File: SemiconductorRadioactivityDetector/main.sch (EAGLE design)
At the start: 32 parts, among them IC1 LM324N, IC2 317T, J1 22-05-7028-02, J2 22-23-2021, J3 22-23-2021, J4 22-23-2021, Q1 2N4093

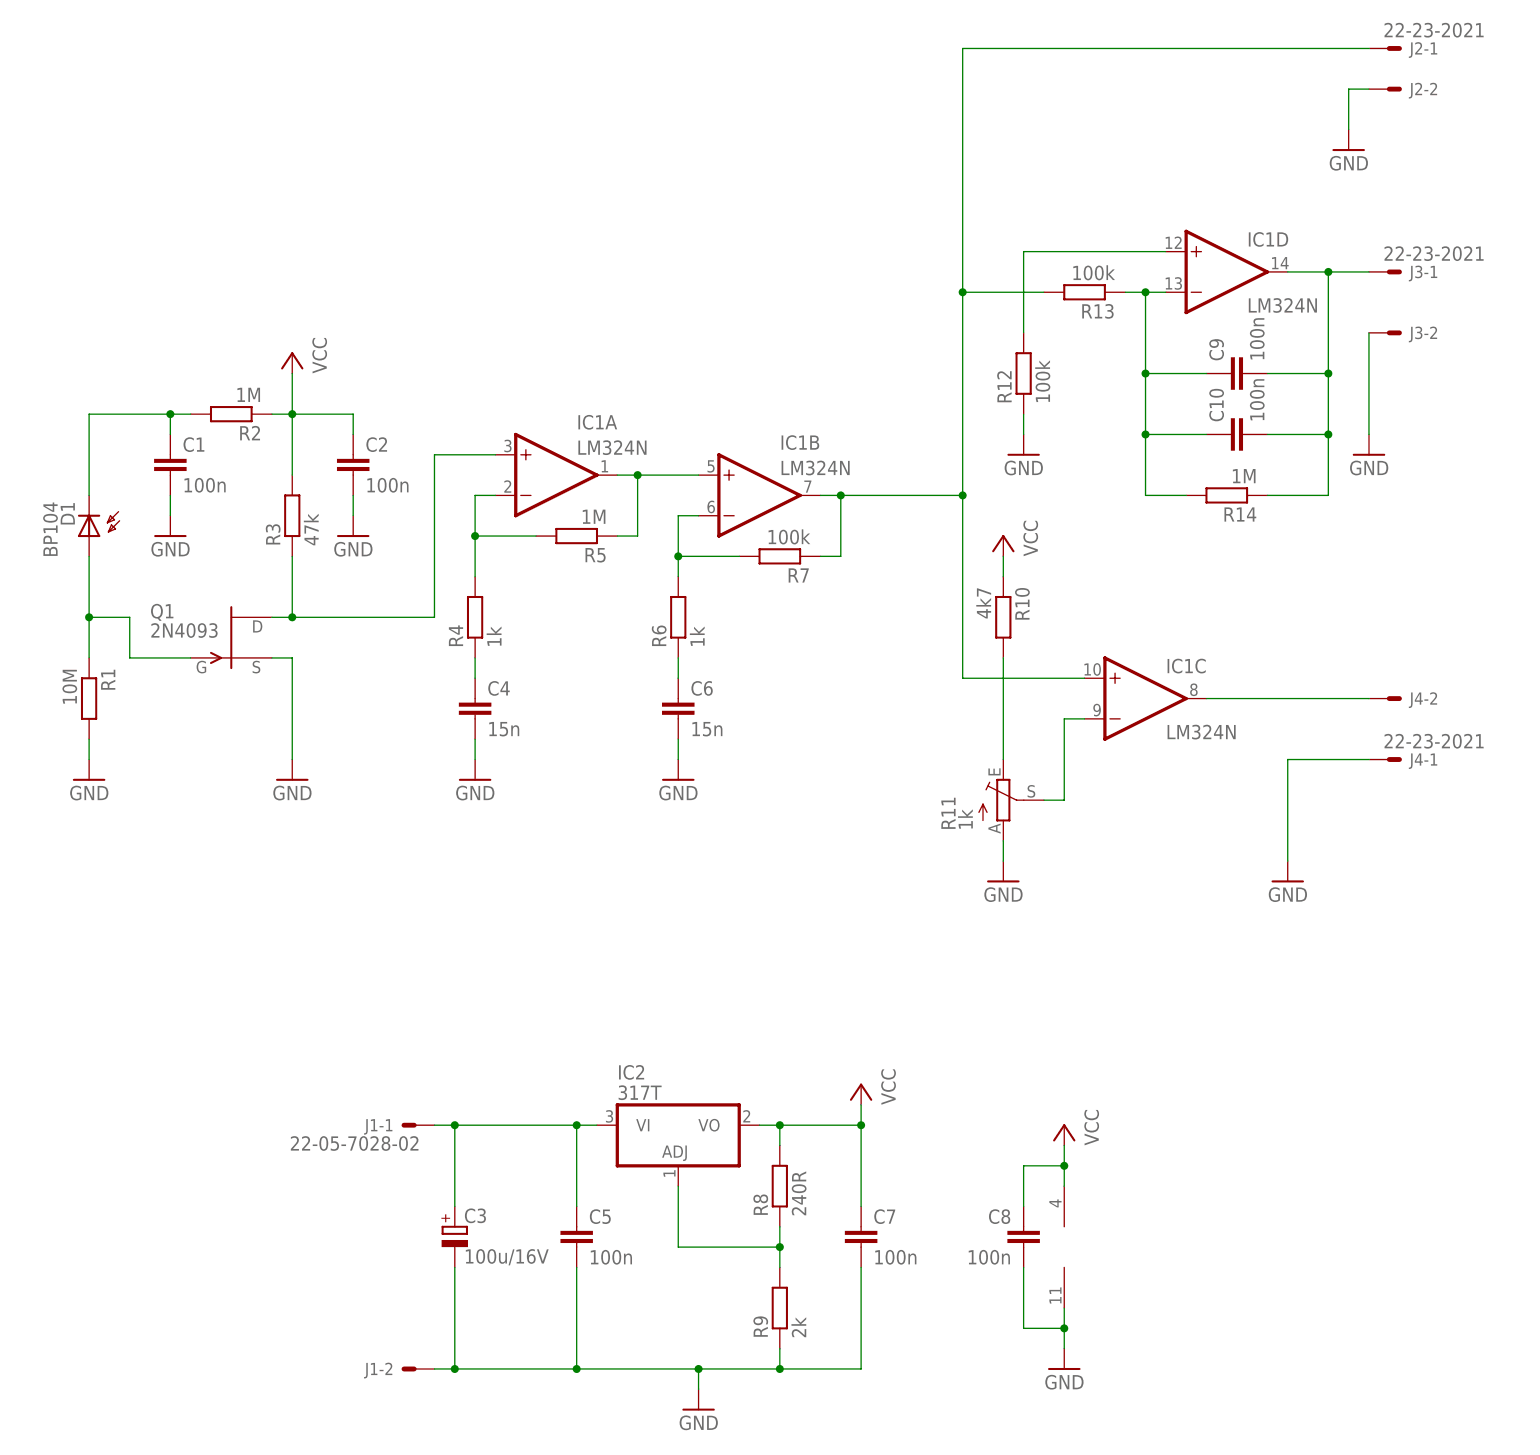
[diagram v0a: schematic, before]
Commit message: Second version. Not working.
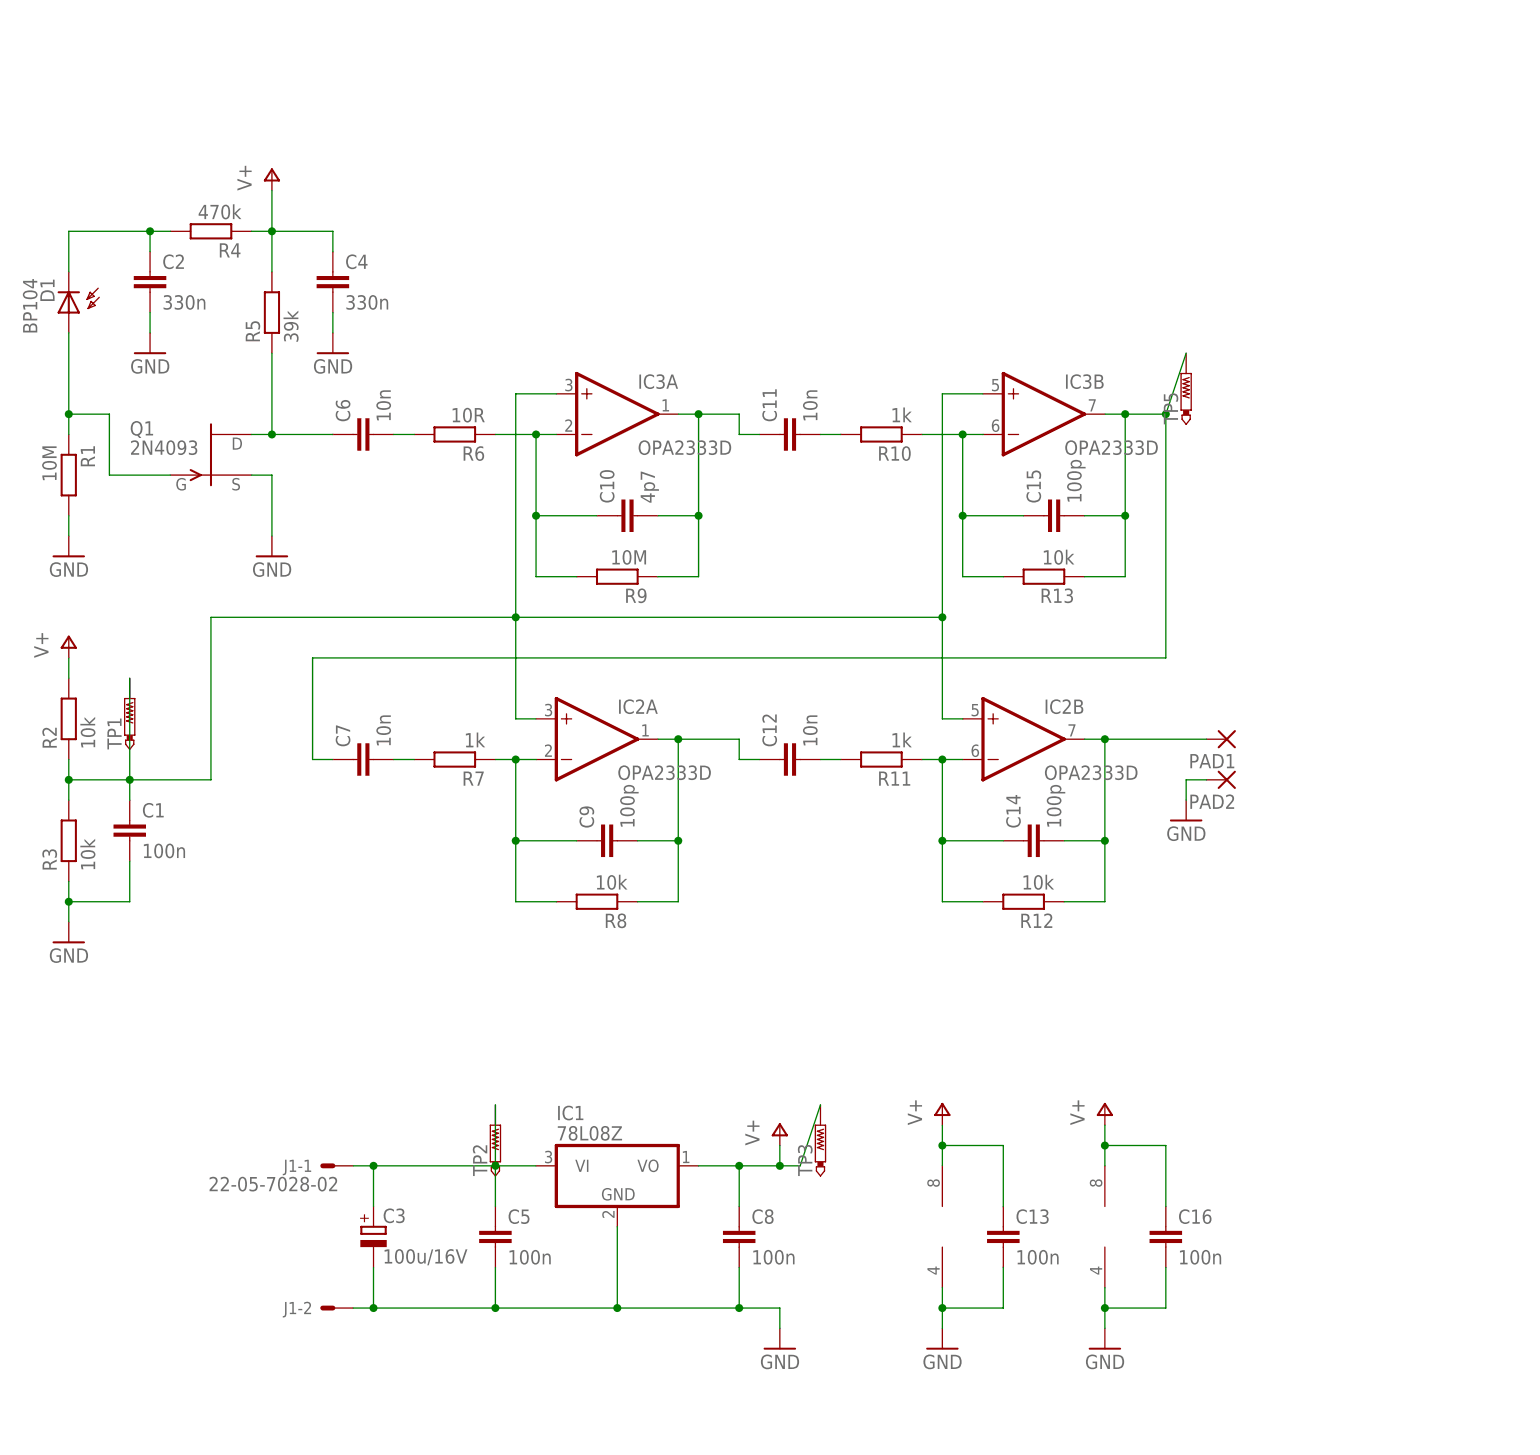
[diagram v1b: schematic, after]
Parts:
- removed J2, J3, J4: 22-23-2021, con-molex:22-23-2021
- removed R14: 1M, resistor:R-EU_M1206
- added C11: 10n, resistor:C-EUC0805
- added C12: 10n, rcl:C-EUC0805
- added C13: 100n, rcl:C-EUC0805
- added C14, C15: 100p, resistor:C-EUC0805
- added C16: 100n, resistor:C-EUC0805
- added IC3: OPA2333D, linear:OPA2333D
- added PAD1, PAD2: (no value), wirepad:1,6/0,8
- added TP1, TP2, TP3, TP5: PTR1TP12R, testpad:PTR1TP12R
- C1, C5, C8: device resistor:C-EUC1206 -> rcl:C-EUC0805
- C10: value 100n -> 4p7; device resistor:C-EUC1206 -> resistor:C-EUC0805
- C2: value 100n -> 330n; device resistor:C-EUC1206 -> rcl:C-EUC0805
- C4: value 15n -> 330n; device resistor:C-EUC1206 -> rcl:C-EUC0805
- C6: value 15n -> 10n; device resistor:C-EUC1206 -> resistor:C-EUC0805
- C7: value 100n -> 10n; device resistor:C-EUC1206 -> resistor:C-EUC0805
- C9: value 100n -> 100p; device resistor:C-EUC1206 -> resistor:C-EUC0805
- IC1: value LM324N -> 78L08Z; device linear:LM324N -> linear:78L08Z
- IC2: value 317T -> OPA2333D; device linear:317T -> linear:OPA2333D
- R10: value 4k7 -> 1k; device resistor:R-EU_M1206 -> rcl:R-EU_R0805
- R11: device pot:TRIM_EU-B64Y -> rcl:R-EU_R0805
- R12: value 100k -> 10k; device resistor:R-EU_R1206 -> rcl:R-EU_R0805
- R13: value 100k -> 10k; device resistor:R-EU_M1206 -> rcl:R-EU_R0805
- R2: value 1M -> 10k; device resistor:R-EU_M1206 -> rcl:R-EU_R0805
- R3: value 47k -> 10k; device resistor:R-EU_M1206 -> rcl:R-EU_R0805
- R4: value 1k -> 470k; device resistor:R-EU_M1206 -> rcl:R-EU_R0805
- R5: value 1M -> 39k; device resistor:R-EU_M1206 -> rcl:R-EU_R0805
- R6: value 1k -> 10R; device resistor:R-EU_M1206 -> rcl:R-EU_R0805
- R7: value 100k -> 1k; device resistor:R-EU_M1206 -> rcl:R-EU_R0805
- R8: value 240R -> 10k; device resistor:R-EU_M1206 -> rcl:R-EU_R0805
- R9: value 2k -> 10M; device resistor:R-EU_M1206 -> rcl:R-EU_0204/2V
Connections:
- removed net N$1: IC2.ADJ, R8.1, R9.2
- removed net N$12: C10.1, C9.1, IC1D.-IN, R13.1, R14.2
- removed net N$18: IC1A.+IN, Q1.D, R3.1
- removed net N$19: IC1B.OUT, IC1C.+IN, J2-1.S, R13.2, R7.1
- removed net N$5: IC1B.-IN, R6.2, R7.2
- removed net VCC: C2.1, C7.1, C8.1, IC1P.V+, IC2.VO, R10.1, R2.1, R3.2, R8.2
- new net N$10: C9.1, IC2A.-IN, R7.1, R8.2
- new net N$20: C10.2, C11.1, IC3A.OUT, R9.1
- new net N$22: C12.1, C9.2, IC2A.OUT, R8.1
- new net N$6: C6.1, Q1.D, R5.1
- new net V+: C13.1, C16.1, C4.1, C8.1, IC1.VO, IC2P.V+, IC3P.V+, R2.2, R4.1, R5.2, TP3.TP
- new net V_REF: C1.1, IC2A.+IN, IC2B.+IN, IC3A.+IN, IC3B.+IN, R2.1, R3.2, TP1.TP
- net GND: now also C13.2, C16.2, IC1.GND, IC2P.V-, IC3P.V-, PAD2.P, R3.1; no longer C6.2, C7.2, IC1P.V-, J2-2.S, J3-2.S, J4-1.S, R11.A, R12.1, R9.1
- net N$11: now also C7.2, R7.2; no longer IC1C.-IN, R11.S
- net N$13: now also C14.1, IC2B.-IN, R11.1, R12.2; no longer C10.2, C9.2, IC1D.OUT, J3-1.S, R14.1
- net N$14: now also C12.2, R11.2; no longer IC1D.+IN, R12.2
- net N$15: now also C11.2, R10.2; no longer IC1C.OUT, J4-2.S
- net N$16: now also C2.1, R4.2; no longer C1.1, R2.2
- net N$2: now also C6.2, R6.2; no longer IC1A.-IN, R4.2, R5.2
- net N$3: now also C14.2, IC2B.OUT, PAD1.P, R12.1; no longer IC1A.OUT, IC1B.+IN, R5.1
- net N$4: now also C10.1, IC3A.-IN, R6.1, R9.2; no longer C4.1, R4.1
- net N$7: now also C15.2, C7.1, IC3B.OUT, R13.1, TP5.TP; no longer C6.1, R6.1
- net N$8: now also IC1.VI, TP2.TP; no longer IC2.VI
- net N$9: now also C15.1, IC3B.-IN, R10.1, R13.2; no longer R10.2, R11.E
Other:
- moved on the sheet: C1, C10, C2, C3, C4, C5, C6, C7, C8, C9, D1, J1-1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

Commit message: Third HW revision, paritialy done.
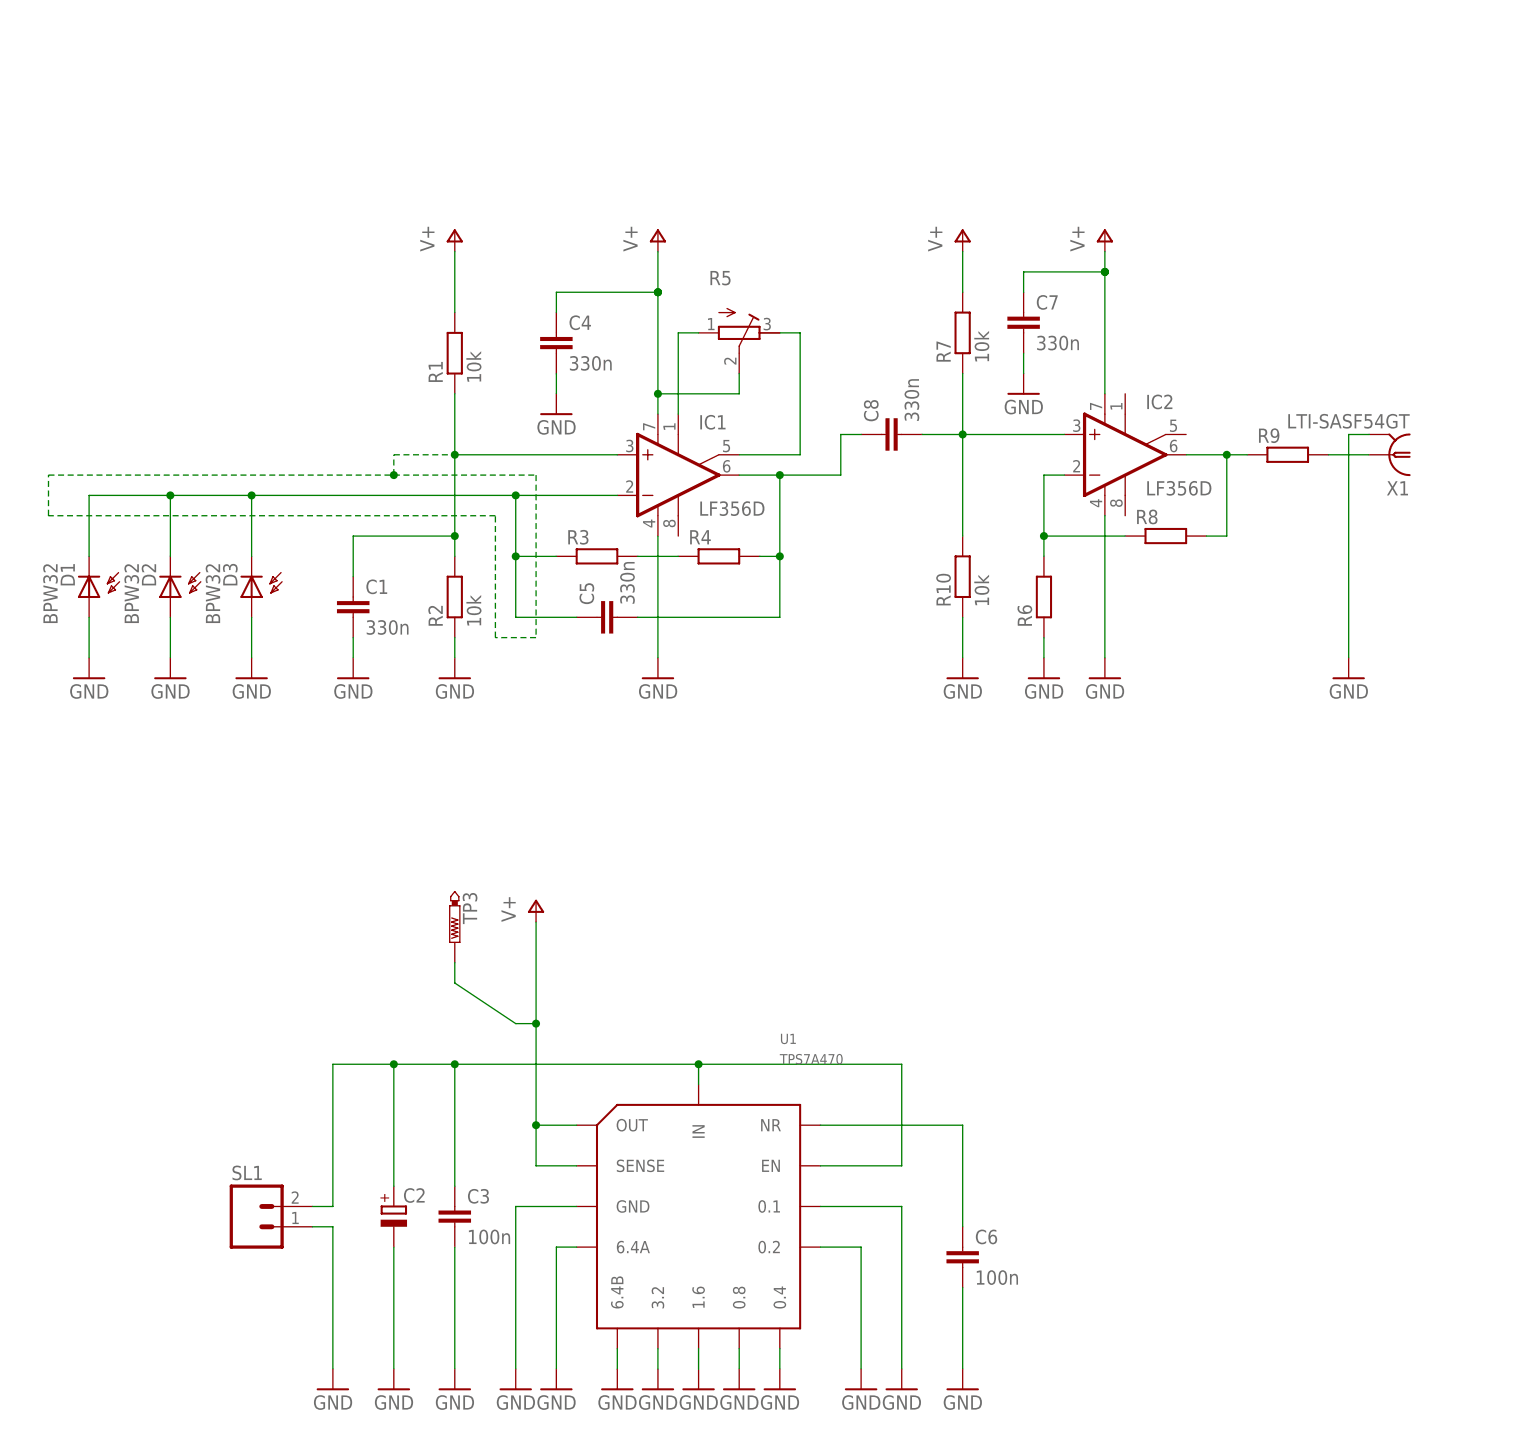
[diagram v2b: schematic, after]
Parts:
- removed C10: 4p7, resistor:C-EUC0805
- removed C11: 10n, resistor:C-EUC0805
- removed C12: 10n, rcl:C-EUC0805
- removed C13: 100n, rcl:C-EUC0805
- removed C14, C15, C9: 100p, resistor:C-EUC0805
- removed C16: 100n, resistor:C-EUC0805
- removed IC3: OPA2333D, linear:OPA2333D
- removed J1: 22-05-7028-02, con-molex:22-05-7028-02
- removed PAD1, PAD2: (no value), wirepad:1,6/0,8
- removed Q1: 2N4093, transistor-fet:2N4093
- removed R11: 1k, rcl:R-EU_R0805
- removed R12, R13: 10k, rcl:R-EU_R0805
- removed TP1, TP2, TP5: PTR1TP12R, testpad:PTR1TP12R
- added D2, D3: BPW32, opto-trans-siemens:BPW32
- added SL1: (no value), con-amp-quick:M02
- added U1: TPS7A470, regulator-jqi:TPS7A470
- added X1: LTI-SASF54GT, con-coax:LTI-SASF54GT
- C1, C5: value 100n -> 330n
- C2: value 330n -> (none); device rcl:C-EUC0805 -> resistor:CPOL-EUT/3528-12R
- C3: value 100u/16V -> 100n; device rcl:CPOL-EU153CLV-0505 -> rcl:C-EUC0805
- C6: value 10n -> 100n; device resistor:C-EUC0805 -> rcl:C-EUC0805
- C7: value 10n -> 330n; device resistor:C-EUC0805 -> rcl:C-EUC0805
- C8: value 100n -> 330n; device rcl:C-EUC0805 -> rcl:C-EUC1206K
- D1: value BP104 -> BPW32; device opto-trans-siemens:BP104 -> opto-trans-siemens:BPW32
- IC1: value 78L08Z -> LF356D; device linear:78L08Z -> linear:LF356D
- IC2: value OPA2333D -> LF356D; device linear:OPA2333D -> linear:LF356D
- R1: value 10M -> 10k; device resistor:R-EU_0204/2V -> rcl:R-EU_R1206
- R10, R7: value 1k -> 10k
- R3: value 10k -> (none); device rcl:R-EU_R0805 -> resistor:R-EU_MELF0204W
- R4: value 470k -> (none); device rcl:R-EU_R0805 -> resistor:R-EU_MELF0204W
- R5: value 39k -> (none); device rcl:R-EU_R0805 -> resistor:R-TRIMM64W
- R6: value 10R -> (none); device rcl:R-EU_R0805 -> resistor:R-EU_M0805
- R8: value 10k -> (none); device rcl:R-EU_R0805 -> resistor:R-EU_M0805
- R9: value 10M -> (none); device rcl:R-EU_0204/2V -> resistor:R-EU_M0805
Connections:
- removed net N$11: C7.2, R7.2
- removed net N$13: C14.1, IC2B.-IN, R11.1, R12.2
- removed net N$16: C2.1, D1.C, R4.2
- removed net N$17: D1.A, Q1.G, R1.1
- removed net N$20: C10.2, C11.1, IC3A.OUT, R9.1
- removed net N$22: C12.1, C9.2, IC2A.OUT, R8.1
- removed net V_REF: C1.1, IC2A.+IN, IC2B.+IN, IC3A.+IN, IC3B.+IN, R2.1, R3.2, TP1.TP
- new net N$1: C5.2, C8.1, IC1.OUT, R4.2
- new net N$5: C6.1, U1.NR
- net GND: now also C2.-, C3.2, C6.2, C7.2, D1.A, D2.A, D3.A, IC1.V-, IC2.V-, R10.1, R2.1, R6.1, SL1.1, U1.0.1, U1.0.2, U1.0.4, U1.0.8, U1.1.6, U1.3.2, U1.6.4A, U1.6.4B, U1.GND, X1.2; no longer C13.2, C16.2, C2.2, C3.-, C5.2, C8.2, IC1.GND, IC2P.V-, IC3P.V-, J1-2.S, PAD2.P, Q1.S, R1.2, R3.1
- net N$10: now also C8.2, IC2.+IN, R10.2; no longer C9.1, IC2A.-IN, R8.2
- net N$14: now also C1.1, IC1.+IN, R1.1, R2.2; no longer C12.2, R11.2
- net N$15: now also R9.2, X1.1; no longer C11.2, R10.2
- net N$2: now also IC2.-IN, R8.1; no longer C6.2
- net N$3: now also R3.2, R4.1; no longer C14.2, IC2B.OUT, PAD1.P, R12.1
- net N$4: now also C5.1, D1.C, D2.C, D3.C, IC1.-IN, R3.1; no longer C10.1, IC3A.-IN, R6.1, R9.2
- net N$6: now also IC1.ON1, R5.A; no longer C6.1, Q1.D, R5.1
- net N$7: now also IC1.ON2, R5.E; no longer C15.2, C7.1, IC3B.OUT, R13.1, TP5.TP
- net N$8: now also C2.+, C3.1, SL1.2, U1.EN, U1.IN; no longer C3.+, C5.1, IC1.VI, J1-1.S, TP2.TP
- net N$9: now also IC2.OUT, R8.2, R9.1; no longer C15.1, IC3B.-IN, R10.1, R13.2
- net V+: now also C7.1, IC1.V+, IC2.V+, R1.2, R5.S, R7.2, U1.OUT, U1.SENSE; no longer C13.1, C16.1, C8.1, IC1.VO, IC2P.V+, IC3P.V+, R2.2, R4.1, R5.2
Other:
- moved on the sheet: C1, C4, C5, C6, C7, C8, D1, R1, R10, R2, R3, R4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
